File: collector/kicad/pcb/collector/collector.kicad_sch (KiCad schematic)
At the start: 1 part, among them U1 ESP32-C6-DevKitC-1

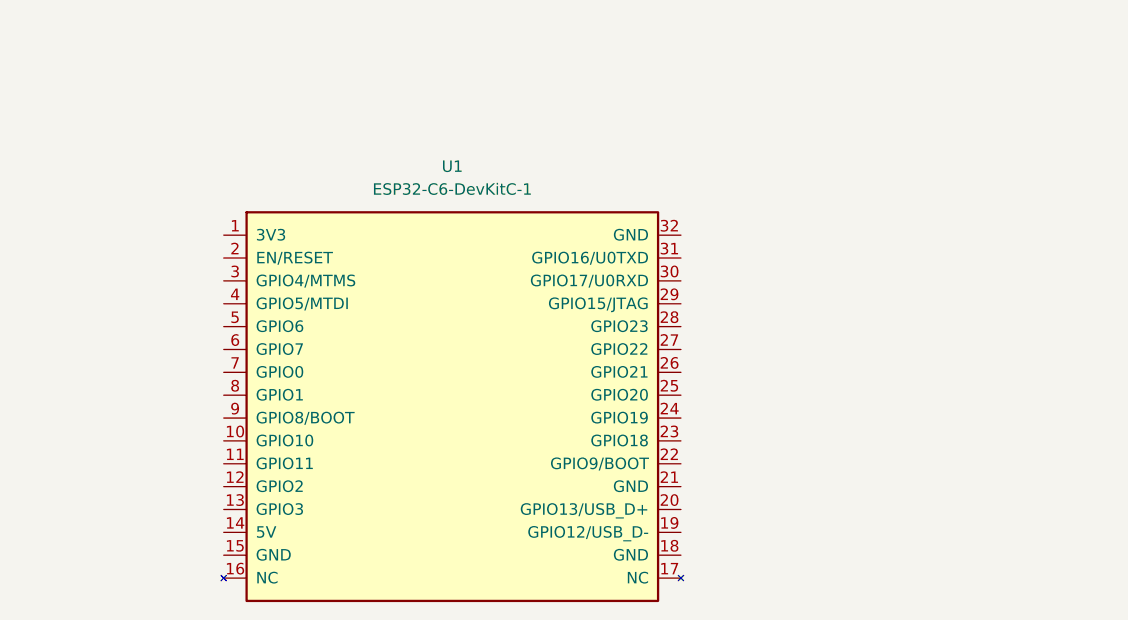
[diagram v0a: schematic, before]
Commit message: keycad first steps
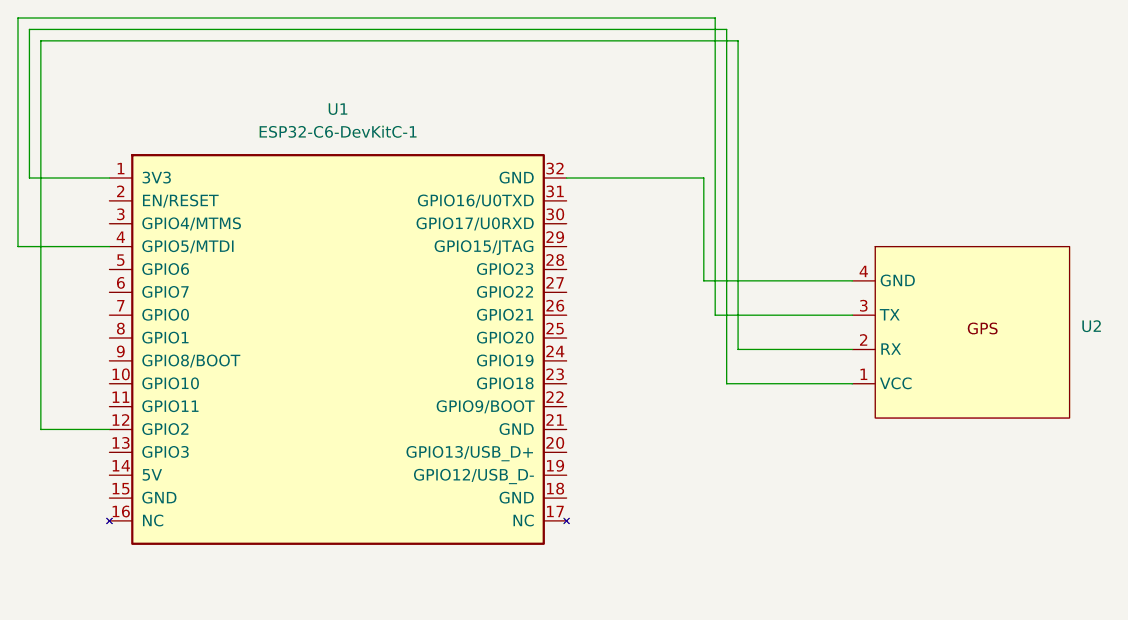
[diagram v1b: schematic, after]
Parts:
- added U2: ~, collector:GY-GPS6MV2, symbol collector:GY-GPS6MV2
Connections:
- net at U1.1 (3V3): now also U2.1 (VCC)
- net at U1.12 (GPIO2): now also U2.2 (RX)
- net at U1.32 (GND): now also U2.4 (GND)
- net at U1.4 (GPIO5/MTDI): now also U2.3 (TX)
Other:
- moved on the sheet: U1
